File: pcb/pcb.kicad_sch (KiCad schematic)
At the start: 232 parts, among them J1 USB_C_Receptacle_USB2.0, J2 AVR-ISP-6, SW1 SW_Push, SW10 SW_Push, SW100 SW_Push, SW101 SW_Push, SW102 SW_Push, SW103 SW_Push, SW104 SW_Push, SW105 SW_Push, SW106 SW_Push, SW107 SW_Push, SW108 SW_Push, SW11 SW_Push, SW12 SW_Push, SW13 SW_Push, SW14 SW_Push, SW15 SW_Push, SW16 SW_Push, SW17 SW_Push, SW18 SW_Push, SW19 SW_Push, SW2 SW_Push, SW20 SW_Push, SW21 SW_Push, SW22 SW_Push, SW23 SW_Push, SW24 SW_Push, SW25 SW_Push, SW26 SW_Push, SW27 SW_Push, SW28 SW_Push, SW29 SW_Push, SW3 SW_Push, SW30 SW_Push, SW31 SW_Push, SW32 SW_Push, SW33 SW_Push, SW34 SW_Push, SW35 SW_Push, SW36 SW_Push, SW37 SW_Push, SW38 SW_Push, SW39 SW_Push, SW4 SW_Push, SW40 SW_Push, SW41 SW_Push, SW42 SW_Push, SW43 SW_Push, SW44 SW_Push, SW45 SW_Push, SW46 SW_Push, SW47 SW_Push, SW48 SW_Push, SW49 SW_Push, SW5 SW_Push, SW50 SW_Push, SW51 SW_Push, SW52 SW_Push, SW53 SW_Push, SW54 SW_Push, SW55 SW_Push, SW56 SW_Push, SW57 SW_Push, SW58 SW_Push, SW59 SW_Push, SW6 SW_Push, SW60 SW_Push, SW61 SW_Push, SW62 SW_Push, SW63 SW_Push, SW64 SW_Push, SW65 SW_Push, SW66 SW_Push, SW67 SW_Push, SW68 SW_Push, SW69 SW_Push, SW7 SW_Push, SW70 SW_Push, SW71 SW_Push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

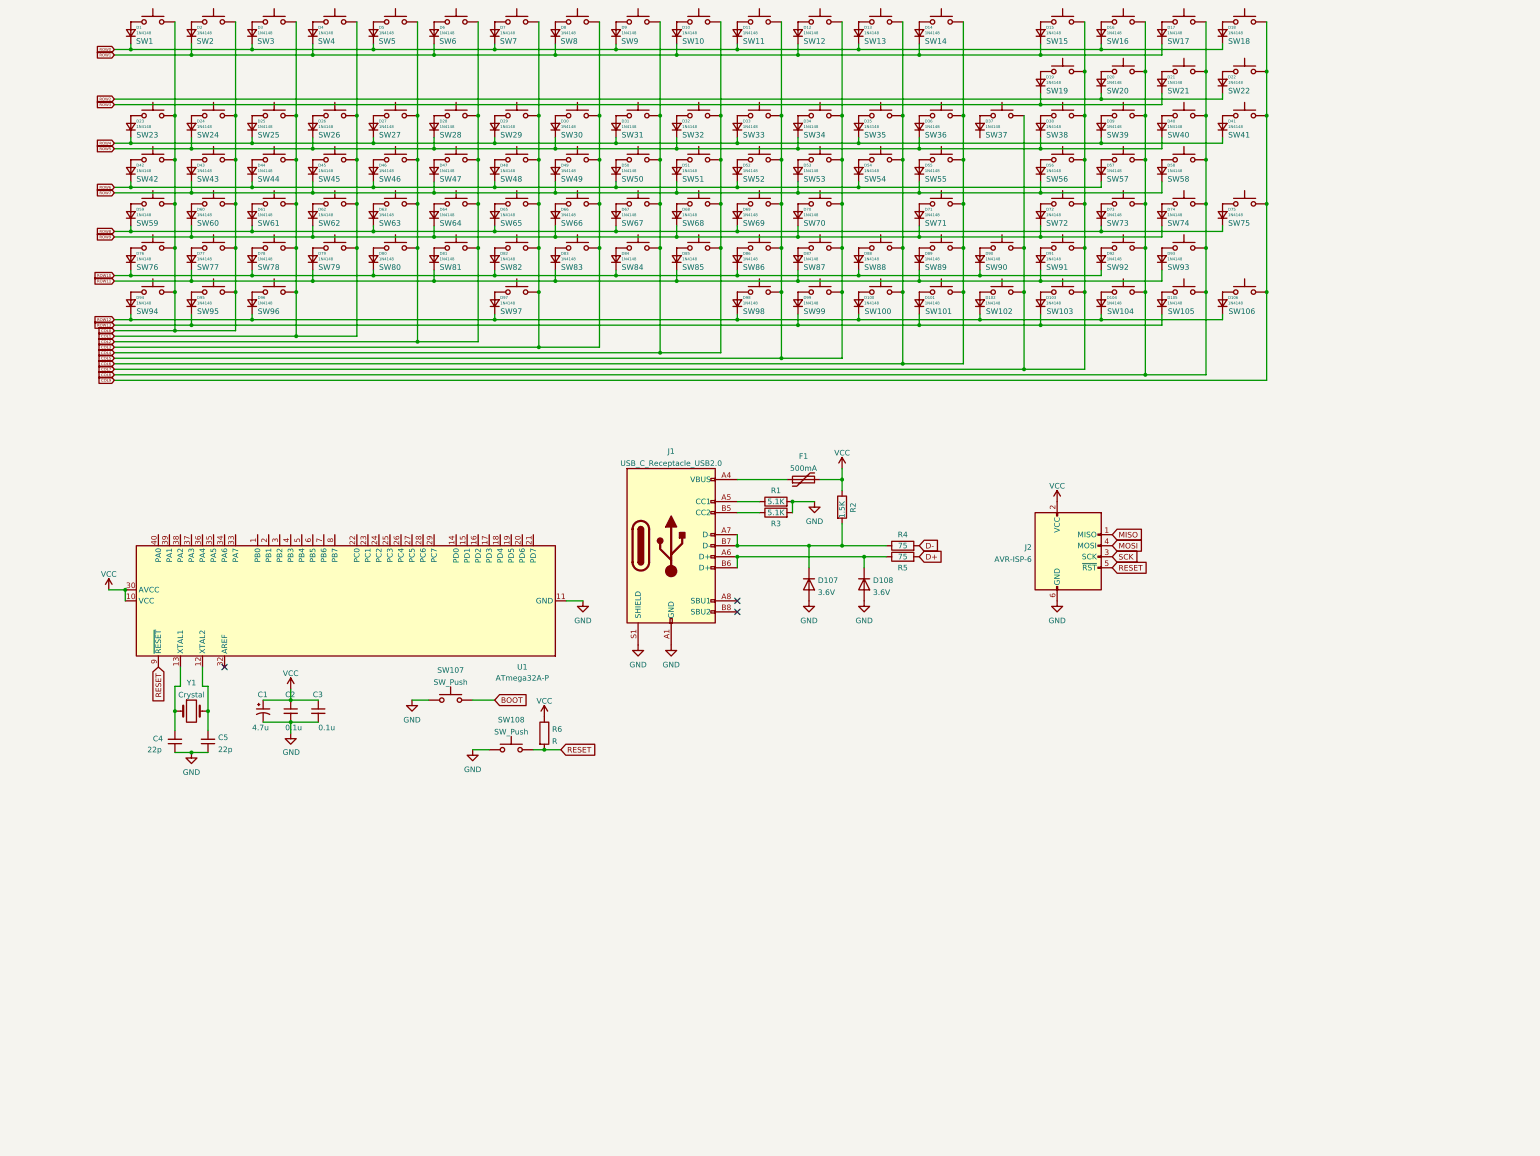
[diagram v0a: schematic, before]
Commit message: Redid wiring on schematic because I hate myself
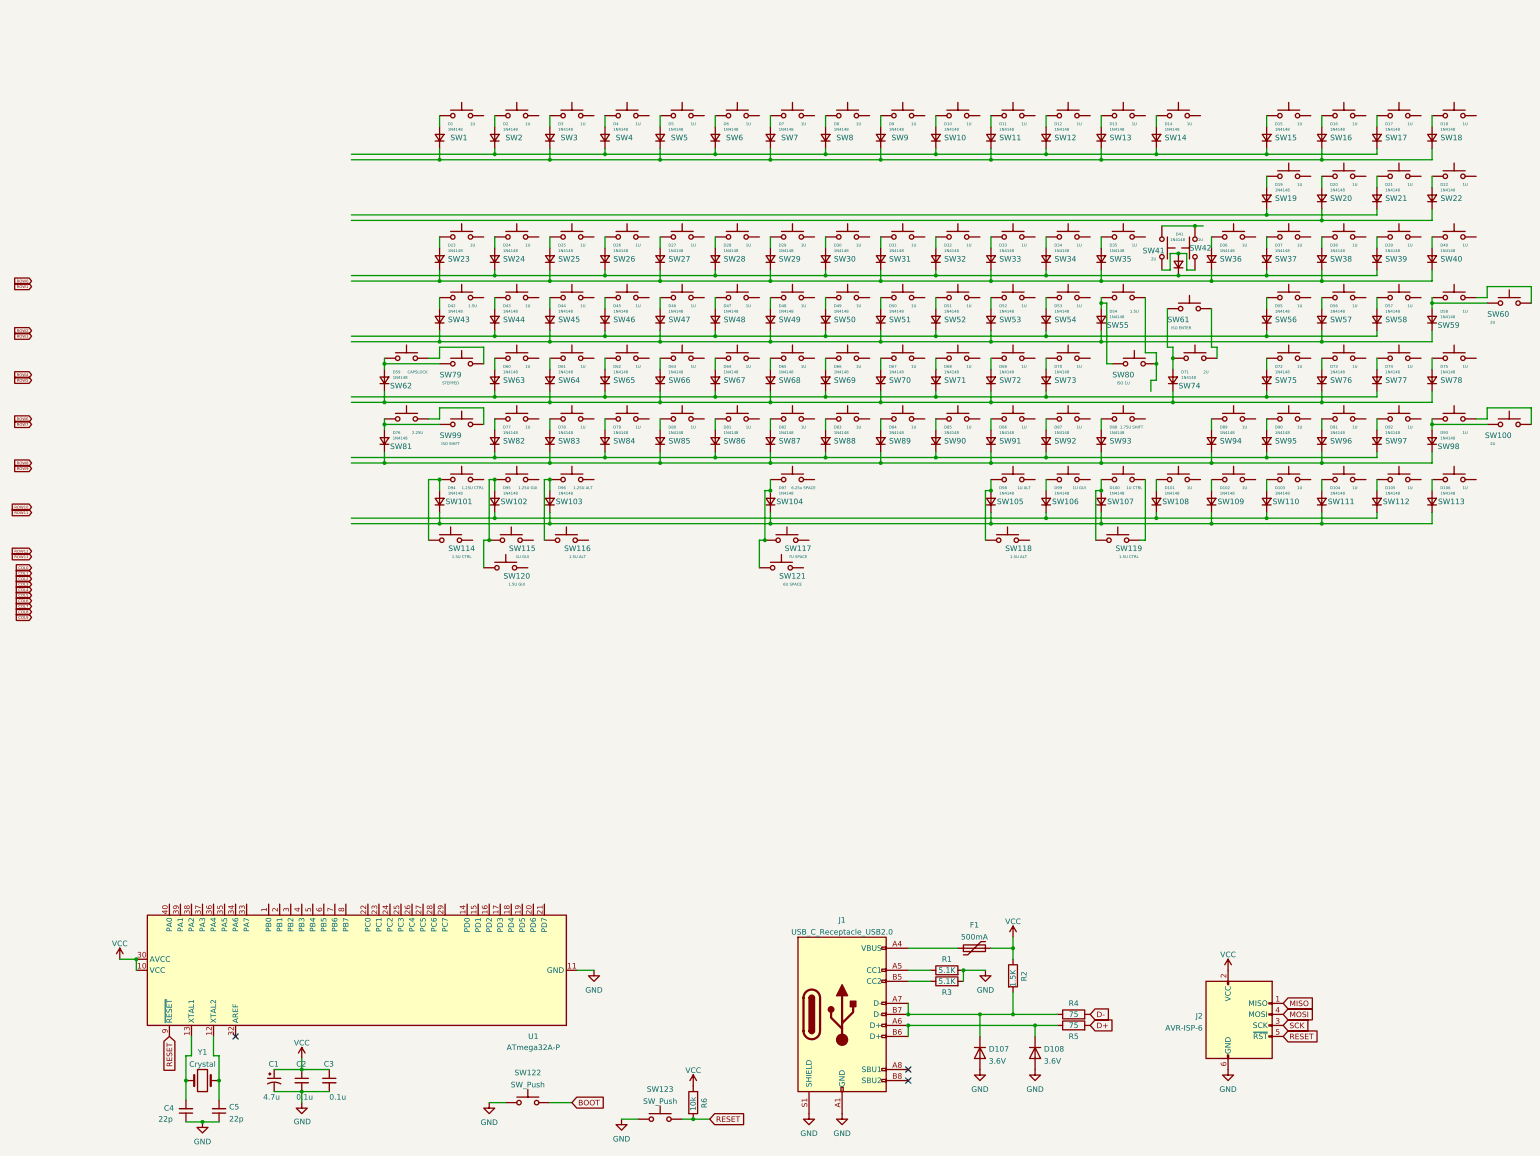
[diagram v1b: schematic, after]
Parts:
- added SW107: 1U CTRL, MX_Only:MXOnly-1U-NoLED, symbol Switch:SW_Push
- added SW108, SW109, SW110, SW111, SW112, SW113: 1U, MX_Only:MXOnly-1U-NoLED, symbol Switch:SW_Push
- added SW114, SW119: 1.5U CTRL, MX_Only:MXOnly-1.5U-NoLED, symbol Switch:SW_Push
- added SW115: 1U GUI, MX_Only:MXOnly-1U-NoLED, symbol Switch:SW_Push
- added SW116, SW118: 1.5U ALT, MX_Only:MXOnly-1.5U-NoLED, symbol Switch:SW_Push
- added SW117: 7U SPACE, MX_Only:MXOnly-7U-NoLED, symbol Switch:SW_Push
- added SW120: 1.5U GUI, MX_Only:MXOnly-1.5U-NoLED, symbol Switch:SW_Push
- added SW121: 6U SPACE, MX_Only:MXOnly-6U-NoLED, symbol Switch:SW_Push
- C1: footprint cftkb:CP_Radial_D4.0mm_P1.50mm -> Capacitor_THT:CP_Radial_D4.0mm_P1.50mm
- C2, C3: footprint cftkb:C_Disc_D4.3mm_W1.9mm_P5.00mm -> Capacitor_THT:C_Disc_D4.3mm_W1.9mm_P5.00mm
- C4, C5: footprint (none) -> Capacitor_THT:C_Disc_D3.0mm_W1.6mm_P2.50mm
- D1, D10, D100, D101, D102, D103, D104, D105, D106, D11, D12, D13, D14, D15, D16, D17, D18, D19, D2, D20, D21, D22, D23, D24, D25, D26, D27, D28, D29, D3, D30, D31, D32, D33, D34, D35, D36, D37, D38, D39, D4, D40, D41, D42, D43, D44, D45, D46, D47, D48, D49, D5, D50, D51, D52, D53, D54, D55, D56, D57, D58, D59, D6, D60, D61, D62, D63, D64, D65, D66, D67, D68, D69, D7, D70, D71, D72, D73, D74, D75, D76, D77, D78, D79, D8, D80, D81, D82, D83, D84, D85, D86, D87, D88, D89, D9, D90, D91, D92, D93, D94, D95, D96, D97, D98, D99: footprint (none) -> Diode_THT:D_DO-35_SOD27_P7.62mm_Horizontal
- D107, D108: footprint (none) -> Diode_THT:D_DO-41_SOD81_P7.62mm_Horizontal
- F1: footprint (none) -> Fuse:Fuse_BelFuse_0ZRE0025FF_L9.6mm_W3.8mm
- J1: footprint (none) -> Connector_USB:USB_C_Receptacle_GCT_USB4085
- J2: footprint (none) -> Connector_PinHeader_2.54mm:PinHeader_2x03_P2.54mm_Vertical
- R1, R2, R3, R4, R5: footprint (none) -> Resistor_THT:R_Axial_DIN0204_L3.6mm_D1.6mm_P7.62mm_Horizontal
- R6: value R -> 10k; footprint (none) -> Resistor_THT:R_Axial_DIN0204_L3.6mm_D1.6mm_P7.62mm_Horizontal
- SW1, SW10, SW11, SW12, SW13, SW14, SW15, SW16, SW17, SW18, SW19, SW2, SW20, SW21, SW22, SW23, SW24, SW25, SW26, SW27, SW28, SW29, SW3, SW30, SW31, SW32, SW33, SW34, SW35, SW36, SW37, SW38, SW39, SW4, SW40, SW42, SW44, SW45, SW46, SW47, SW48, SW49, SW5, SW50, SW51, SW52, SW53, SW54, SW56, SW57, SW58, SW59, SW6, SW63, SW64, SW65, SW66, SW67, SW68, SW69, SW7, SW70, SW71, SW72, SW73, SW75, SW76, SW77, SW78, SW8, SW82, SW83, SW84, SW85, SW86, SW87, SW88, SW89, SW9, SW90, SW91, SW92, SW94, SW95, SW96, SW97, SW98: value SW_Push -> 1U; footprint (none) -> MX_Only:MXOnly-1U-NoLED
- SW100, SW41, SW60, SW74: value SW_Push -> 2U; footprint (none) -> MX_Only:MXOnly-2U-NoLED
- SW101: value SW_Push -> 1.25U CTRL; footprint (none) -> MX_Only:MXOnly-1.25U-NoLED
- SW102: value SW_Push -> 1.25U GUI; footprint (none) -> MX_Only:MXOnly-1.25U-NoLED
- SW103: value SW_Push -> 1.25U ALT; footprint (none) -> MX_Only:MXOnly-1.25U-NoLED
- SW104: value SW_Push -> 6.25u SPACE; footprint (none) -> MX_Only:MXOnly-6.25U-NoLED
- SW105: value SW_Push -> 1U ALT; footprint (none) -> MX_Only:MXOnly-1U-NoLED
- SW106: value SW_Push -> 1U GUI; footprint (none) -> MX_Only:MXOnly-1U-NoLED
- SW122: renamed from SW107; footprint (none) -> Button_Switch_THT:SW_PUSH_6mm_H5mm
- SW123: renamed from SW108; footprint (none) -> Button_Switch_THT:SW_PUSH_6mm_H5mm
- SW43, SW55: value SW_Push -> 1.5U; footprint (none) -> MX_Only:MXOnly-1.5U-NoLED
- SW61: value SW_Push -> ISO ENTER; footprint (none) -> MX_Only:MXOnly-ISO-NoLED
- SW62: value SW_Push -> CAPSLOCK; footprint (none) -> MX_Only:MXOnly-1.75U-NoLED
- SW79: value SW_Push -> STEPPED; footprint (none) -> MX_Only:MXOnly-1.25U-NoLED
- SW80: value SW_Push -> ISO 1U; footprint (none) -> MX_Only:MXOnly-1U-NoLED
- SW81: value SW_Push -> 2.25U; footprint (none) -> MX_Only:MXOnly-2.25U-NoLED
- SW93: value SW_Push -> 1.75U SHIFT; footprint (none) -> MX_Only:MXOnly-1.75U-NoLED
- SW99: value SW_Push -> ISO SHIFT; footprint (none) -> MX_Only:MXOnly-1.25U-NoLED
- Y1: footprint (none) -> Crystal:Crystal_HC49-4H_Vertical
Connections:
- net COL0: no longer SW1.2, SW2.2, SW23.2, SW24.2, SW42.2, SW43.2, SW59.2, SW60.2, SW76.2, SW77.2, SW94.2, SW95.2
- net COL1: no longer SW25.2, SW26.2, SW3.2, SW4.2, SW44.2, SW45.2, SW61.2, SW62.2, SW78.2, SW79.2, SW96.2
- net COL2: no longer SW27.2, SW28.2, SW46.2, SW47.2, SW5.2, SW6.2, SW63.2, SW64.2, SW80.2, SW81.2
- net COL3: no longer SW29.2, SW30.2, SW48.2, SW49.2, SW65.2, SW66.2, SW7.2, SW8.2, SW82.2, SW83.2, SW97.2
- net COL4: no longer SW10.2, SW31.2, SW32.2, SW50.2, SW51.2, SW67.2, SW68.2, SW84.2, SW85.2, SW9.2
- net COL5: no longer SW11.2, SW12.2, SW33.2, SW34.2, SW52.2, SW53.2, SW69.2, SW70.2, SW86.2, SW87.2, SW98.2, SW99.2
- net COL6: no longer SW100.2, SW101.2, SW13.2, SW14.2, SW35.2, SW36.2, SW54.2, SW55.2, SW71.2, SW88.2, SW89.2
- net COL7: no longer SW102.2, SW103.2, SW15.2, SW19.2, SW37.2, SW38.2, SW56.2, SW72.2, SW90.2, SW91.2
- net COL8: no longer SW104.2, SW105.2, SW16.2, SW17.2, SW20.2, SW21.2, SW39.2, SW40.2, SW57.2, SW58.2, SW73.2, SW74.2, SW92.2, SW93.2
- net COL9: no longer SW106.2, SW18.2, SW22.2, SW41.2, SW75.2
- net ROW0: no longer D1.1 (K), D11.1 (K), D13.1 (K), D16.1 (K), D18.1 (K), D3.1 (K), D5.1 (K), D7.1 (K), D9.1 (K)
- net ROW1: no longer D10.1 (K), D12.1 (K), D14.1 (K), D15.1 (K), D17.1 (K), D2.1 (K), D4.1 (K), D6.1 (K), D8.1 (K)
- net ROW10: no longer D76.1 (K), D78.1 (K), D80.1 (K), D82.1 (K), D84.1 (K), D86.1 (K), D88.1 (K), D90.1 (K), D92.1 (K)
- net ROW11: no longer D77.1 (K), D79.1 (K), D81.1 (K), D83.1 (K), D85.1 (K), D87.1 (K), D89.1 (K), D91.1 (K), D93.1 (K)
- net ROW12: no longer D100.1 (K), D102.1 (K), D104.1 (K), D106.1 (K), D94.1 (K), D96.1 (K), D97.1 (K), D98.1 (K)
- net ROW13: no longer D101.1 (K), D103.1 (K), D105.1 (K), D95.1 (K), D99.1 (K)
- net ROW2: no longer D20.1 (K), D22.1 (K)
- net ROW3: no longer D19.1 (K), D21.1 (K)
- net ROW4: no longer D23.1 (K), D25.1 (K), D27.1 (K), D29.1 (K), D31.1 (K), D33.1 (K), D35.1 (K), D39.1 (K), D41.1 (K)
- net ROW5: no longer D24.1 (K), D26.1 (K), D28.1 (K), D30.1 (K), D32.1 (K), D34.1 (K), D36.1 (K), D38.1 (K), D40.1 (K)
- net ROW6: no longer D42.1 (K), D44.1 (K), D46.1 (K), D48.1 (K), D50.1 (K), D52.1 (K), D54.1 (K), D57.1 (K)
- net ROW7: no longer D43.1 (K), D45.1 (K), D47.1 (K), D49.1 (K), D51.1 (K), D53.1 (K), D55.1 (K), D56.1 (K), D58.1 (K)
- net ROW8: no longer D59.1 (K), D61.1 (K), D63.1 (K), D65.1 (K), D67.1 (K), D69.1 (K), D73.1 (K), D75.1 (K)
- net ROW9: no longer D60.1 (K), D62.1 (K), D64.1 (K), D66.1 (K), D68.1 (K), D70.1 (K), D71.1 (K), D72.1 (K), D74.1 (K)
- net at D77.2 (A): now also SW82.1; no longer SW77.1
- net at SW70.1: now also D67.2 (A); no longer D70.2 (A)
- net at SW65.1: now also D62.2 (A); no longer D65.2 (A)
- net at D43.2 (A): now also SW44.1; no longer SW43.1
- net at SW98.1: now also D93.2 (A), SW100.1; no longer D98.2 (A)
- net at D95.2 (A): now also SW102.1, SW115.1, SW120.1; no longer SW95.1
- net at SW74.1: now also D71.2 (A), SW61.1; no longer D74.2 (A)
- net at D82.2 (A): now also SW87.1; no longer SW82.1
- net at D45.2 (A): now also SW46.1; no longer SW45.1
- net at D91.2 (A): now also SW96.1; no longer SW91.1
- net at SW66.1: now also D63.2 (A); no longer D66.2 (A)
- net at D56.2 (A): now also SW57.1; no longer SW56.1
- net at SW52.1: now also D51.2 (A); no longer D52.2 (A)
- net at SW84.1: now also D79.2 (A); no longer D84.2 (A)
- net at SW92.1: now also D87.2 (A); no longer D92.2 (A)
- net at SW79.1: now also D59.2 (A), SW62.1; no longer D79.2 (A)
- net at SW94.1: now also D89.2 (A); no longer D94.2 (A)
- net at D69.2 (A): now also SW72.1; no longer SW69.1
- net at SW47.1: now also D46.2 (A); no longer D47.2 (A)
- net at D76.2 (A): now also SW81.1, SW99.1; no longer SW76.1
- net at SW60.1: now also D58.2 (A), SW59.1; no longer D60.2 (A)
- net at D96.2 (A): now also SW103.1, SW116.1; no longer SW96.1
- net at D72.2 (A): now also SW75.1; no longer SW72.1
- net at D99.2 (A): now also SW106.1; no longer SW99.1
- net at D73.2 (A): now also SW76.1; no longer SW73.1
- net at D105.2 (A): now also SW112.1; no longer SW105.1
- net at SW88.1: now also D83.2 (A); no longer D88.2 (A)
- net at SW78.1: now also D75.2 (A); no longer D78.2 (A)
- net at SW68.1: now also D65.2 (A); no longer D68.2 (A)
- net at SW89.1: now also D84.2 (A); no longer D89.2 (A)
- net at SW93.1: now also D88.2 (A); no longer D93.2 (A)
- net at D49.2 (A): now also SW50.1; no longer SW49.1
- net at D61.2 (A): now also SW64.1; no longer SW61.1
- net at SW71.1: now also D68.2 (A); no longer D71.2 (A)
- net at SW101.1: now also D94.2 (A), SW114.1; no longer D101.2 (A)
- net at D81.2 (A): now also SW86.1; no longer SW81.1
- net at SW63.1: now also D60.2 (A); no longer D63.2 (A)
- net at D100.2 (A): now also SW107.1, SW119.1; no longer SW100.1
- net at SW90.1: now also D85.2 (A); no longer D90.2 (A)
- net at SW48.1: now also D47.2 (A); no longer D48.2 (A)
- net at D102.2 (A): now also SW109.1; no longer SW102.1
- net at SW80.1: now also D54.2 (A), SW55.1; no longer D80.2 (A)
- net at SW85.1: now also D80.2 (A); no longer D85.2 (A)
- net at D44.2 (A): now also SW45.1; no longer SW44.1
- net at SW54.1: now also D53.2 (A); no longer D54.2 (A)
- net at SW83.1: now also D78.2 (A); no longer D83.2 (A)
- net at SW42.1: now also D41.2 (A), SW41.2; no longer D42.2 (A)
- net at D55.2 (A): now also SW56.1; no longer SW55.1
- net at SW51.1: now also D50.2 (A); no longer D51.2 (A)
- net at SW58.1: now also D57.2 (A); no longer D58.2 (A)
- net at D86.2 (A): now also SW91.1; no longer SW86.1
- net at D103.2 (A): now also SW110.1; no longer SW103.1
- net at SW67.1: now also D64.2 (A); no longer D67.2 (A)
- net at SW53.1: now also D52.2 (A); no longer D53.2 (A)
- net at D97.2 (A): now also SW104.1, SW117.1, SW121.1; no longer SW97.1
- net at D37.1 (K): now also D24.1 (K), D26.1 (K), D28.1 (K), D30.1 (K), D32.1 (K), D34.1 (K), D39.1 (K), D41.1 (K)
- net at D106.2 (A): now also SW113.1; no longer SW106.1
- net at SW41.1: now also SW42.2; no longer D41.2 (A)
- net at D104.2 (A): now also SW111.1; no longer SW104.1
- new net: D1.1 (K), D11.1 (K), D13.1 (K), D16.1 (K), D18.1 (K), D3.1 (K), D5.1 (K), D7.1 (K), D9.1 (K)
- new net: SW100.2, SW98.2
- new net: D76.1 (K), D78.1 (K), D80.1 (K), D82.1 (K), D84.1 (K), D86.1 (K), D88.1 (K), D89.1 (K), D91.1 (K), D93.1 (K)
- new net: D23.1 (K), D25.1 (K), D27.1 (K), D29.1 (K), D31.1 (K), D33.1 (K), D35.1 (K), D36.1 (K), D38.1 (K), D40.1 (K)
- new net: SW61.2, SW74.2
- new net: D77.1 (K), D79.1 (K), D81.1 (K), D83.1 (K), D85.1 (K), D87.1 (K), D90.1 (K), D92.1 (K)
- new net: SW59.2, SW60.2
- new net: D101.1 (K), D103.1 (K), D105.1 (K), D95.1 (K), D99.1 (K)
- new net: D42.1 (K), D44.1 (K), D46.1 (K), D48.1 (K), D50.1 (K), D52.1 (K), D54.1 (K), D56.1 (K), D58.1 (K)
- new net: D100.1 (K), D102.1 (K), D104.1 (K), D106.1 (K), D94.1 (K), D96.1 (K), D97.1 (K), D98.1 (K)
- new net: SW62.2, SW79.2
- new net: D10.1 (K), D12.1 (K), D14.1 (K), D15.1 (K), D17.1 (K), D2.1 (K), D4.1 (K), D6.1 (K), D8.1 (K)
- new net: SW81.2, SW99.2
- new net: D19.1 (K), D21.1 (K)
- new net: D59.1 (K), D61.1 (K), D63.1 (K), D65.1 (K), D67.1 (K), D69.1 (K), D71.1 (K), D73.1 (K), D75.1 (K)
- new net: D20.1 (K), D22.1 (K)
- new net: SW107.2, SW119.2
- new net: D60.1 (K), D62.1 (K), D64.1 (K), D66.1 (K), D68.1 (K), D70.1 (K), D72.1 (K), D74.1 (K)
- new net: D70.2 (A), SW73.1
- new net: SW55.2, SW80.2
- new net: D43.1 (K), D45.1 (K), D47.1 (K), D49.1 (K), D51.1 (K), D53.1 (K), D55.1 (K), D57.1 (K)
- new net: D92.2 (A), SW97.1
- new net: D90.2 (A), SW95.1
- new net: D42.2 (A), SW43.1
- new net: D74.2 (A), SW77.1
- new net: D101.2 (A), SW108.1
- new net: D98.2 (A), SW105.1, SW118.1
- new net: D66.2 (A), SW69.1
- new net: D48.2 (A), SW49.1
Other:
- moved on the sheet: C1, C2, C3, C4, C5, D107, D108, F1, J1, J2, R1, R2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
